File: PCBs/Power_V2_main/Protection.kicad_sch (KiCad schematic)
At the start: 22 parts, among them J10 TYPE-C-31-M-12, J12 Conn_01x02, J18 YK4420203000G, J2 Conn_01x02, J3 Conn_01x02, Q4 NTD25P03LT4G, U4 178.6164.0001, U5 TVS3300DRV, U9 AMS1117-3.3

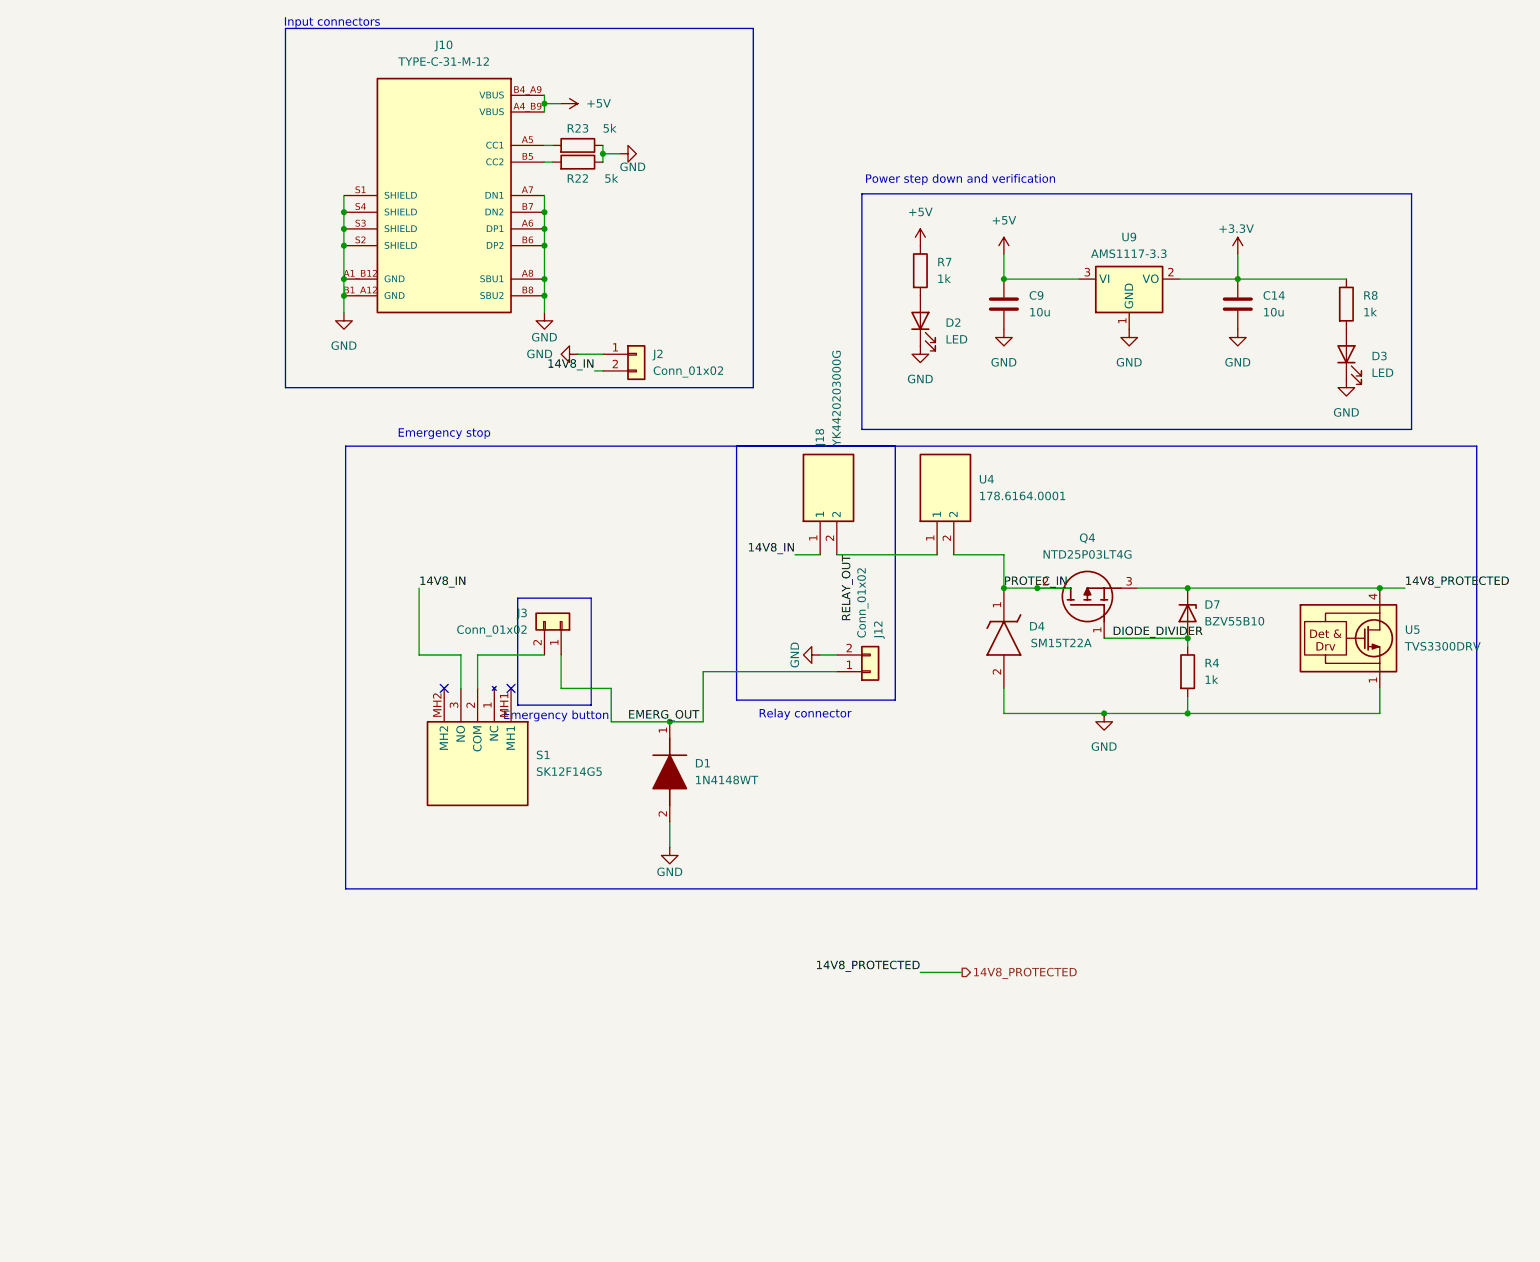
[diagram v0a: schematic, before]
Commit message: a 5 hour binge of PCB layout on the main
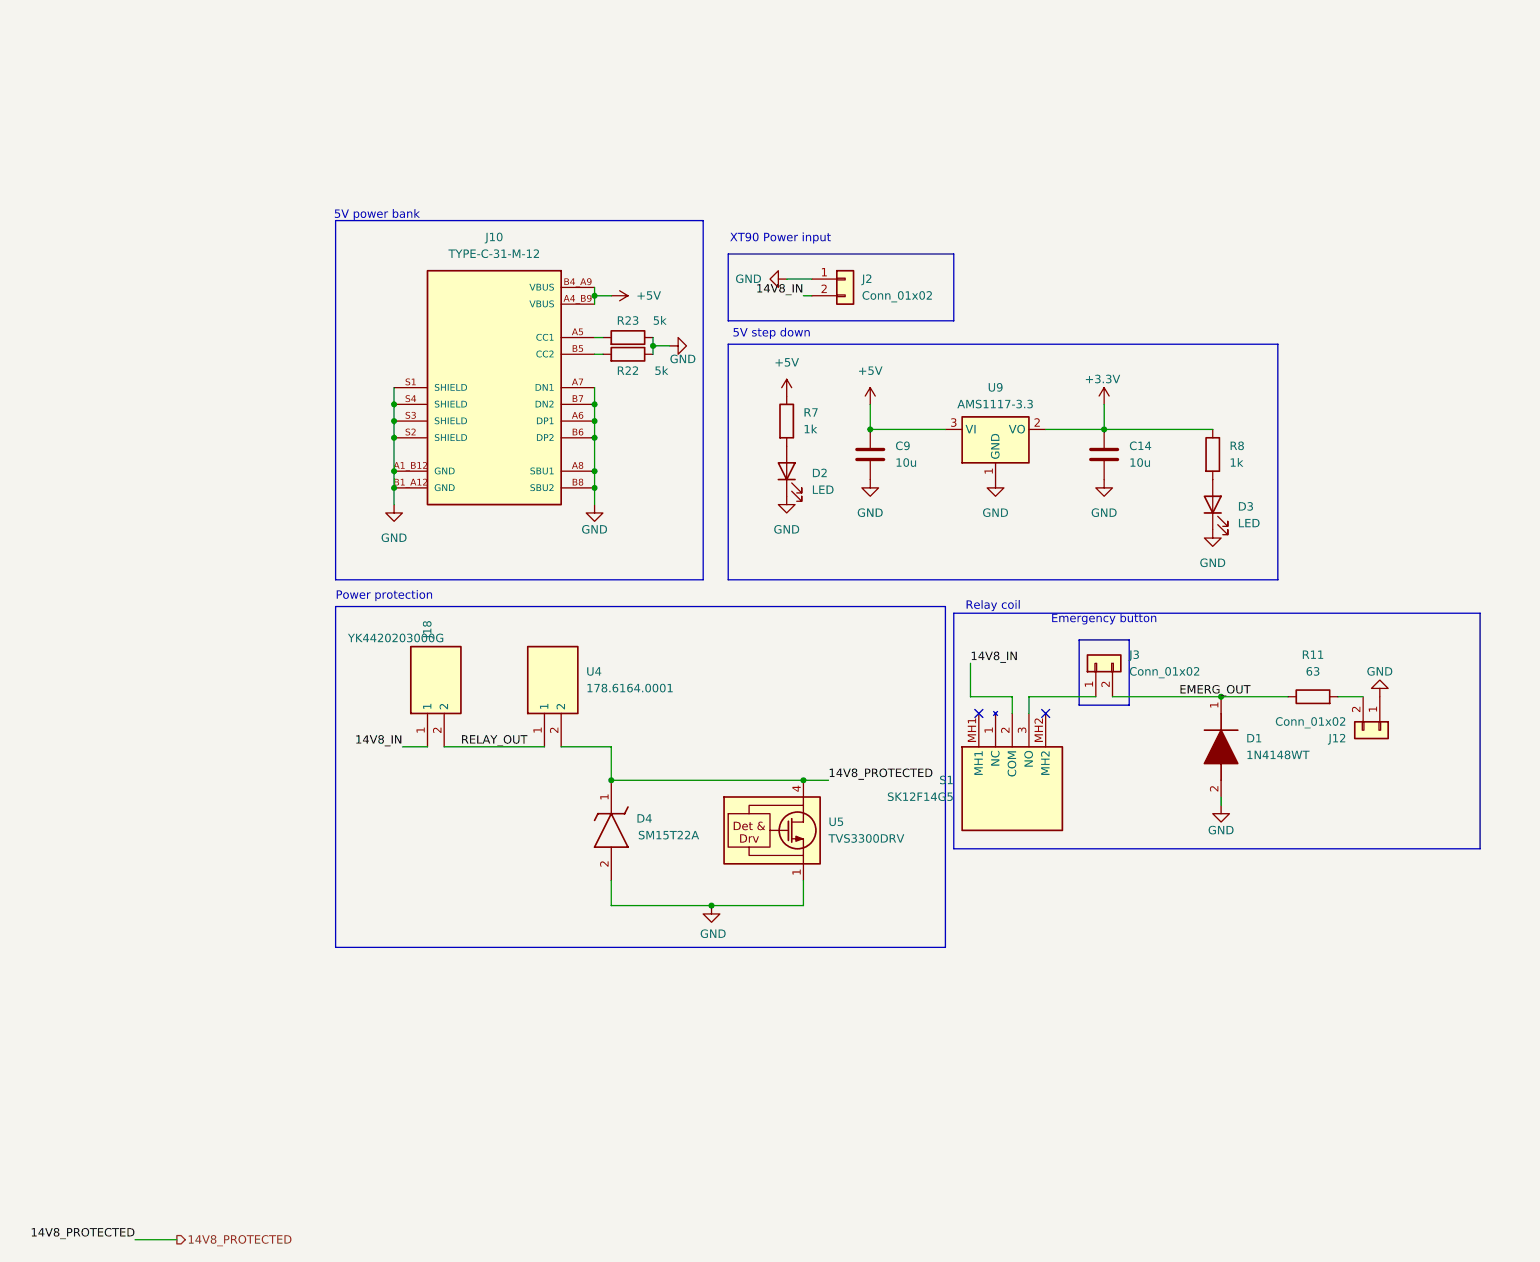
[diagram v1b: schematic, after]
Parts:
- removed D7: BZV55B10, Diode_SMD:D_MiniMELF, symbol Diode:BZV55B10
- removed Q4: NTD25P03LT4G, iprl_footprints:MJD45H11T4G, symbol NTD25P03LT4G:NTD25P03LT4G
- removed R4: 1k, Resistor_SMD:R_0805_2012Metric, symbol Device:R
- added R11: 63, Resistor_SMD:R_0805_2012Metric, symbol Device:R
- S1: footprint IPRL_footprints:SK12F14G5 -> iprl_footprints:SK12F14G5
- U4: footprint IPRL_footprints:178.6164.XXX1 -> iprl_footprints:178.6164.XXX1
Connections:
- net PROTEC_IN is gone; now on net 14V8_PROTECTED: D4.1 (K), U4.2
- net 14V8_IN: now also S1.2 (COM); no longer S1.3 (NO)
- net EMERG_OUT: now also J3.2 (Pin_2), R11.1; no longer J12.1 (Pin_1), J3.1 (Pin_1)
- net GND: now also J12.1 (Pin_1); no longer J12.2 (Pin_2)
- new net: J3.1 (Pin_1), S1.3 (NO)
- new net: J12.2 (Pin_2), R11.2
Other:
- note added: "5V power bank"
- note added: "5V step down"
- note added: "Power protection"
- note added: "Relay coil"
- note added: "XT90 Power input"
- note removed: "Emergency stop"
- note removed: "Input connectors"
- note removed: "Power step down and verification"
- note removed: "Relay connector"
- moved on the sheet: C14, C9, D1, D2, D3, D4, J10, J12, J18, J2, J3, R22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
